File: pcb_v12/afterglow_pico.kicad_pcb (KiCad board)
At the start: 2 copper layers, 57.5 x 57.5 mm, 40 parts, among them J1 Conn_02x17_Odd_Even, J2 Conn_02x17_Odd_Even, U1 74LS21, U2 7408, U3 SN74LVC245AN, U4 SN74LVC245AN, U5 SC0915, U6 74LS245, U7 74LS245, U8 74LS257, U9 74LS257

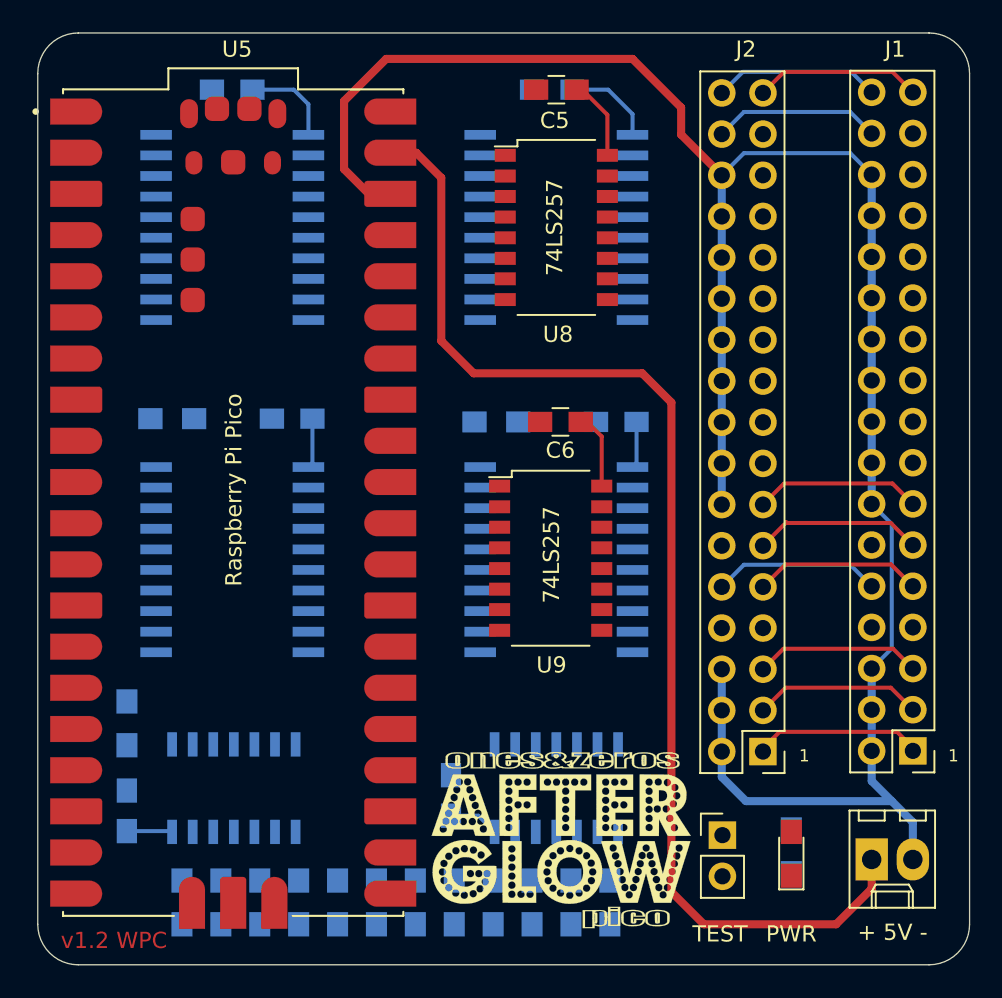
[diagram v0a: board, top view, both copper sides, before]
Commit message: Routing preparations
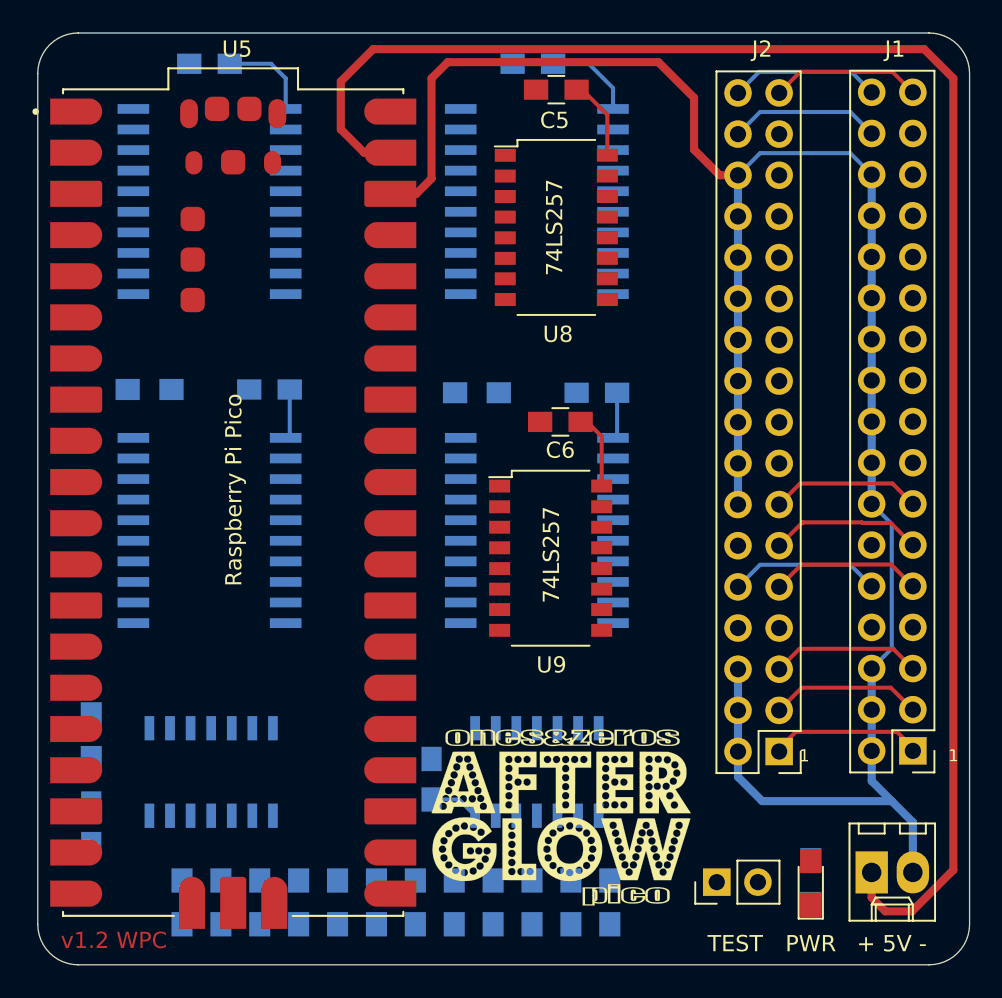
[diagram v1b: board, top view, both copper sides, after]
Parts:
- moved TEST 2.92 mm to (209.4, 117.4), turned to 90 degrees
- moved R16 2.34 mm to (170.8, 108.4)
- moved C8 2.34 mm to (170.8, 113.8)
- moved R5 2.28 mm to (174.4, 87.0)
- moved U7 2.28 mm to (178.1, 95.7)
- moved C4 2.28 mm to (181.8, 87.0)
- moved R3 2.25 mm to (215.2, 117.4)
- moved R2 2.16 mm to (194.6, 87.2)
- moved C2 2.16 mm to (202.0, 87.2)
- moved PWR 2.16 mm to (215.2, 117.5)
- moved U4 2.16 mm to (198.3, 95.7)
- moved C3 2.13 mm to (178.1, 66.9)
- moved U6 2.13 mm to (178.1, 75.4)
- moved C1 2.00 mm to (198.1, 66.9)
- moved U3 2.00 mm to (198.3, 75.4)
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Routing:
- net +5V: track 100.2 -> 124.5 mm
- net GND: track 128.8 -> 124.8 mm
- net /SOL4: track 10.4 -> 9.36 mm
- net /ZERO_CROSS: track 10.3 -> 9.31 mm
- net /TRIAC: track 10.3 -> 9.31 mm
- net /SOL2: track 10.4 -> 9.38 mm
- net /P33: track 10.3 -> 9.31 mm
- net /DIS3: track 10.4 -> 9.36 mm
- net /DIS2: track 10.4 -> 9.39 mm
- net /DIS1: track 10.3 -> 9.28 mm
- net /DIS_STROBE: track 10.5 -> 9.47 mm
- net /SOL3: track 10.4 -> 9.48 mm

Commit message: PCB v1.2 routed
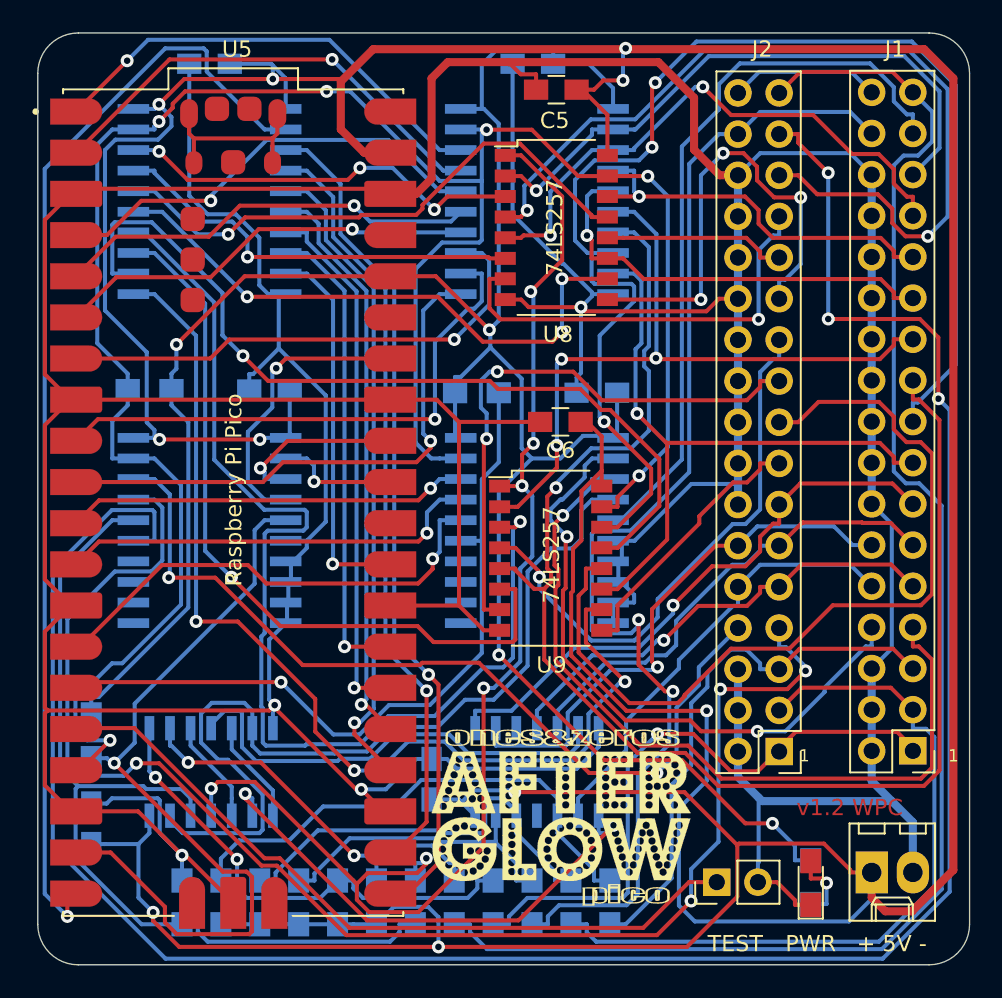
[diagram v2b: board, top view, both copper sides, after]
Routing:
- net GND: track 124.8 -> 439.6 mm, vias 0 -> 4
- net +5V: track 124.5 -> 323.3 mm, vias 0 -> 10
- net /PICO_BLANK: track 0.00 -> 143.0 mm, vias 0 -> 3
- net /PICO_EN_OUT: track 0.00 -> 138.0 mm, vias 0 -> 6
- net +3V3: track 8.49 -> 140.8 mm, vias 0 -> 4
- net /LROW_PICO: track 0.00 -> 89.1 mm, vias 0 -> 4
- net /D5: track 0.00 -> 88.9 mm, vias 0 -> 1
- net /P33: track 9.31 -> 94.7 mm
- net /D6: track 0.00 -> 82.2 mm, vias 0 -> 3
- net /OUT_SEL: track 0.00 -> 80.4 mm, vias 0 -> 6
- net Net-(U5-Pad20): track 0.00 -> 69.1 mm, vias 0 -> 1
- net /D4_PICO: track 0.00 -> 68.0 mm, vias 0 -> 1
- net /DIS3: track 9.36 -> 75.8 mm, vias 0 -> 2
- net /D7_PICO: track 0.00 -> 64.8 mm, vias 0 -> 3
- net /COMB_EV: track 0.00 -> 54.7 mm
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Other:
- board text removed: "v1.1 WPC"
